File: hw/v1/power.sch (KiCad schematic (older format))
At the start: 24 parts, among them J502 USB_C_Receptacle, J601 Screw_Terminal, J602 USB_B_Micro, Q604 Q_PMOS_GSD, Q605 Q_PMOS_GSD, U602 FUSB302BMPX

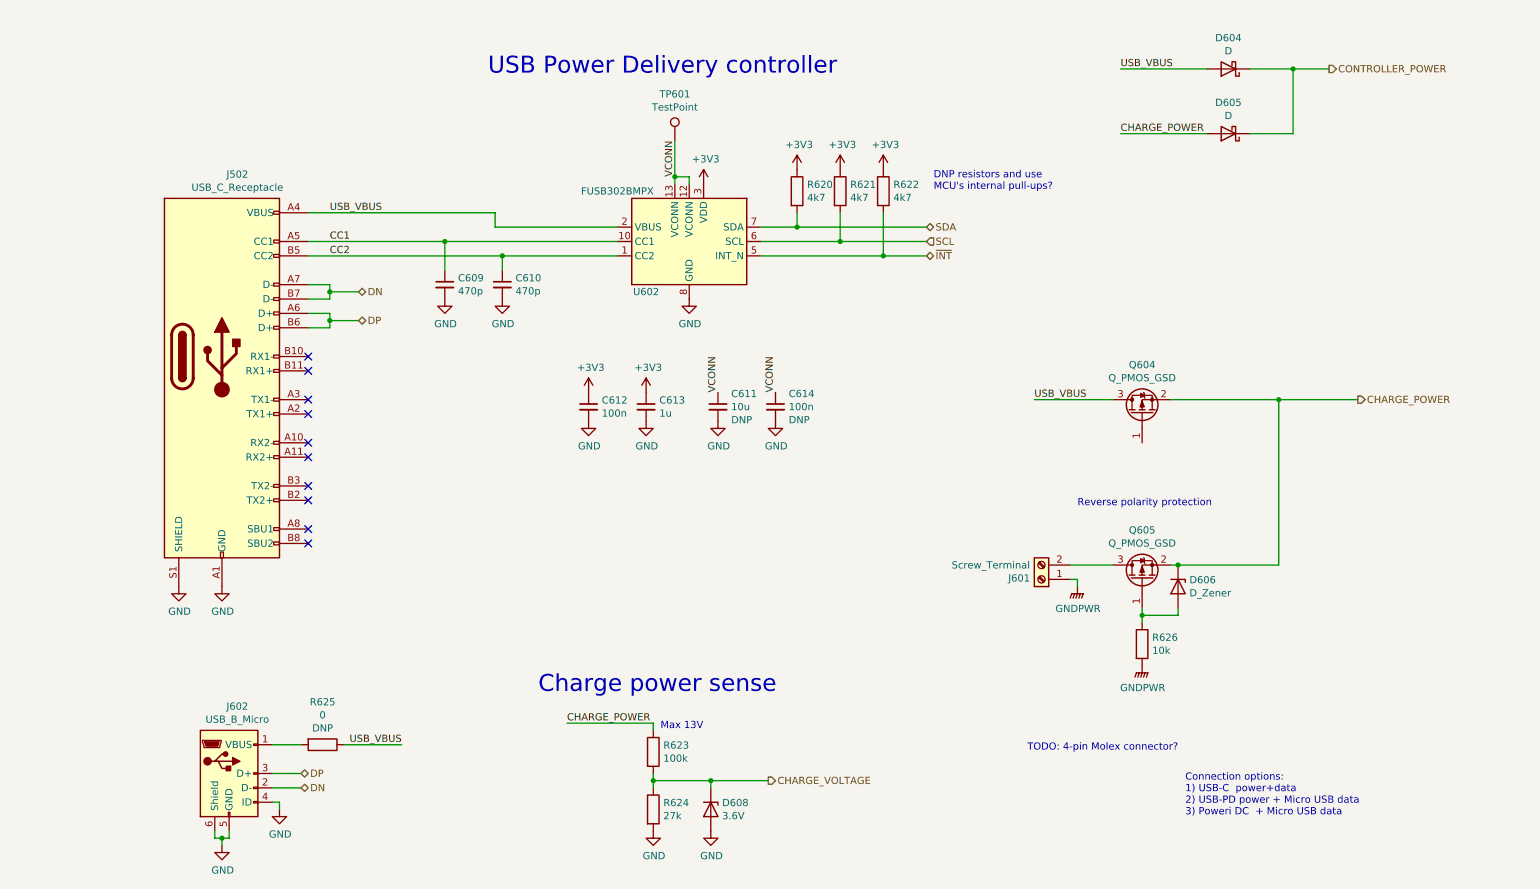
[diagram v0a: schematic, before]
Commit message: Soon...
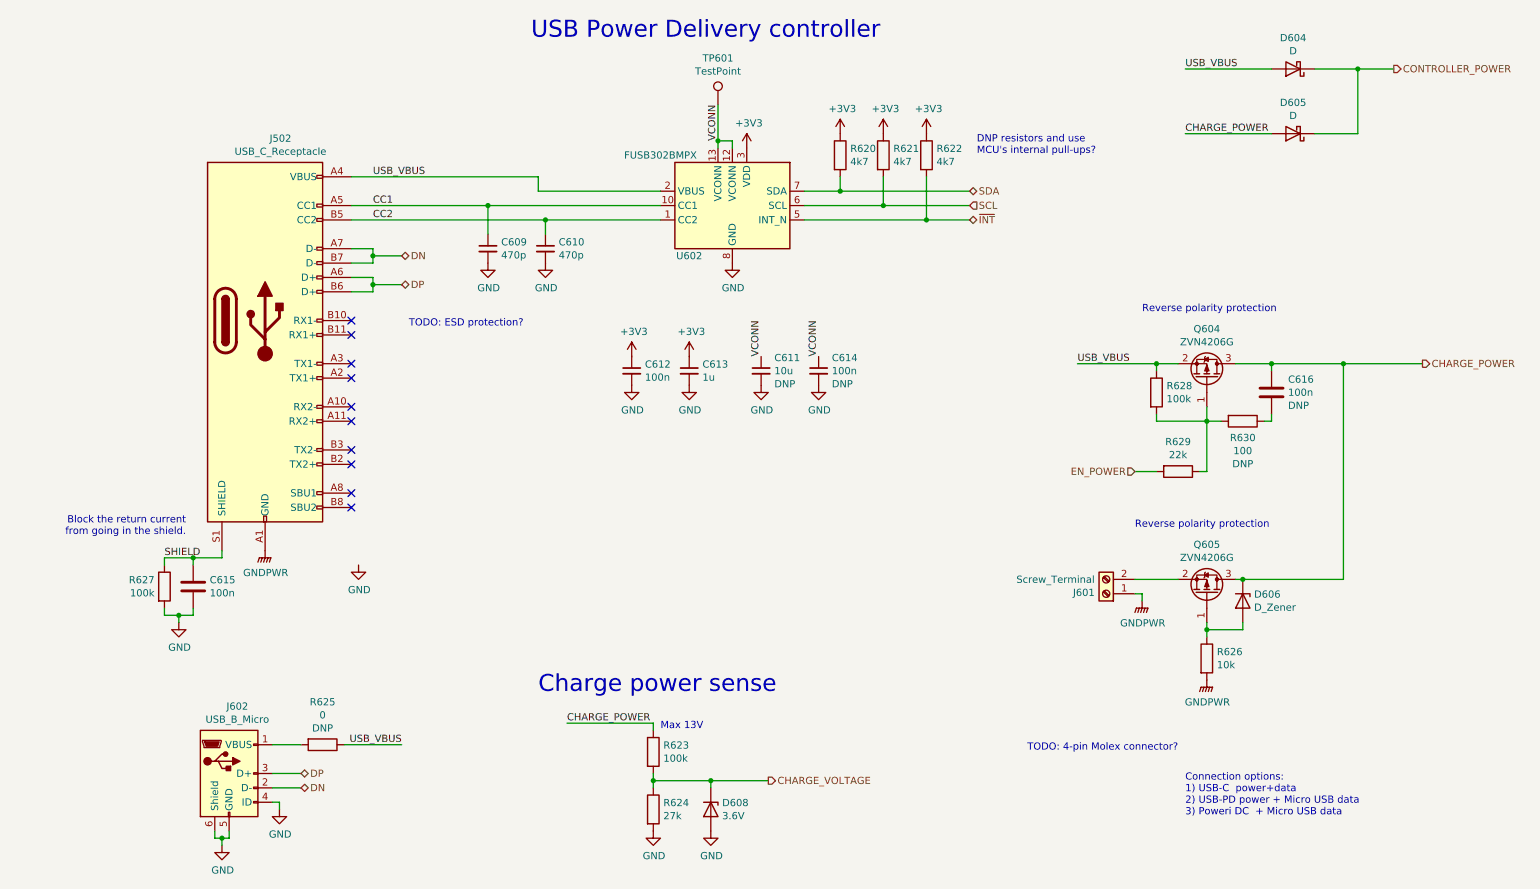
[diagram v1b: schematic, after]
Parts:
- added C615, C616: 100n, Capacitor_SMD:C_0603_1608Metric, symbol Device:C
- added R627, R628: 100k, Resistor_SMD:R_0603_1608Metric, symbol Device:R
- added R629: 22k, Resistor_SMD:R_0603_1608Metric, symbol Device:R
- added R630: 100, Resistor_SMD:R_0603_1608Metric, symbol Device:R
- D606: footprint (none) -> Diode_SMD:D_SOD-123
- Q604, Q605: value Q_PMOS_GSD -> ZVN4206G; footprint (none) -> Package_TO_SOT_SMD:SOT-223-3_TabPin2
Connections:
- net CHARGE_POWER: now also Q604.3 (D), Q605.3 (D), C616.1; no longer Q604.2 (S), Q605.2 (S)
- net GND: now also C615.2, R627.2; no longer J502.A1 (GND), J502.A12 (GND), J502.B1 (GND), J502.B12 (GND), J502.S1 (SHIELD)
- net GNDPWR: now also J502.A1 (GND), J502.A12 (GND), J502.B1 (GND), J502.B12 (GND)
- net USB_VBUS: now also Q604.2 (S), R628.1; no longer Q604.3 (D)
- net at J601.2 (Pin_2): now also Q605.2 (S); no longer Q605.3 (D)
- net at Q604.1 (G): now also R628.2, R629.1, R630.2
- new net: C616.2, R630.1
- new net EN_POWER: R629.2
- new net SHIELD: C615.1, J502.S1 (SHIELD), R627.1
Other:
- note added: "Block the return current\nfrom going in the shield."
- note added: "TODO: ESD protection?"
- moved on the sheet: C609, C610, C611, C612, C613, C614, D604, D605, D606, J502, J601, Q604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
